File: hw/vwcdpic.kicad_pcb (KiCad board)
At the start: 2 copper layers, 14.6 x 13.1 mm, 12 parts, among them U1 PIC12F629, U2 LM78L05ACZ, U3 MC78L05ACH

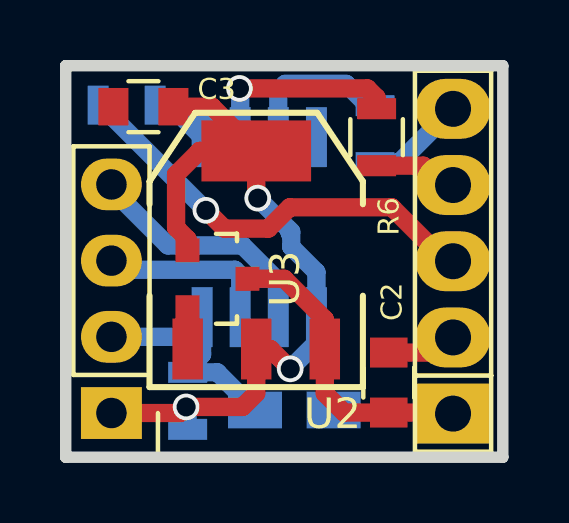
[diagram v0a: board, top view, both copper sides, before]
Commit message: update
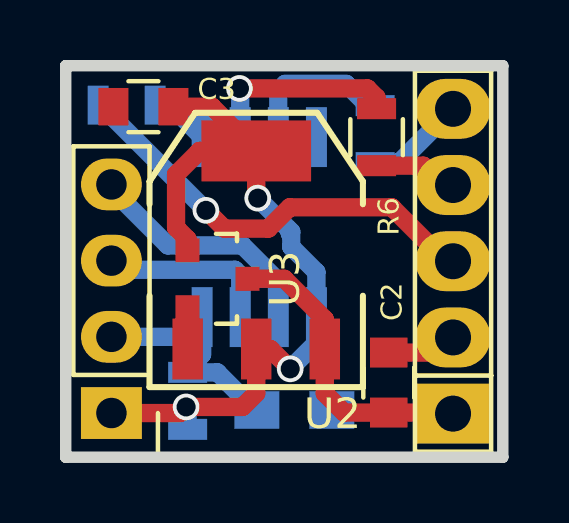
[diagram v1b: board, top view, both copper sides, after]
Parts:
- C1: value 1uF/6.3V -> 1uF/16V; footprint Capacitors_Tantalum_SMD:TantalC_SizeA_EIA-3216_Reflow -> Capacitors_SMD:C_0805_HandSoldering
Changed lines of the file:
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@@
-(kicad_pcb (version 4) (host pcbnew 0.201510080346+6253~30~ubuntu14.04.1-product)
+(kicad_pcb (version 4) (host pcbnew 0.201511080416+6302~30~ubuntu14.04.1-product)
   (general
     (links 26)
@@
       (net 10 ARCHOS))
   )
-  (module Capacitors_Tantalum_SMD:TantalC_SizeA_EIA-3216_Reflow (layer Back)
-    (at 145.3896 125.8824)
-    (descr "Tantal Cap. , Size A, EIA-3216, Reflow")
-    (tags "Tantal Capacitor Size-A EIA-3216 reflow")
-    (attr smd)
-    (fp_text reference C1 (at 2.2352 -1.6764 180) (layer B.SilkS)
-      (effects (font (size 0.7 0.7) (thickness 0.1)) (justify mirror))
-    )
-    (fp_text value 1uF/6.3V (at 0 -2.1) (layer B.Fab) hide
-      (effects (font (size 1 1) (thickness 0.15)) (justify mirror))
-    )
-    (fp_line (start 1.6 -0.9) (end -2.1 -0.9) (layer B.SilkS) (width 0.15))
-    (fp_line (start 1.6 0.9) (end -2.1 0.9) (layer B.SilkS) (width 0.15))
-    (fp_line (start -2.5 -1.2) (end 2.5 -1.2) (layer B.CrtYd) (width 0.05))
-    (fp_line (start 2.5 -1.2) (end 2.5 1.2) (layer B.CrtYd) (width 0.05))
-    (fp_line (start 2.5 1.2) (end -2.5 1.2) (layer B.CrtYd) (width 0.05))
-    (fp_line (start -2.5 1.2) (end -2.5 -1.2) (layer B.CrtYd) (width 0.05))
-    (pad 2 smd rect (at 1.31 0) (size 1.8 1.23) (layers Back B.Paste B.Mask)
-      (net 2 GND))
-    (pad 1 smd rect (at -1.31 0) (size 1.8 1.23) (layers Back B.Paste B.Mask)
-      (net 8 RESET))
-    (model Capacitors_Tantalum_SMD.3dshapes/TantalC_SizeA_EIA-3216_Reflow.wrl
-      (at (xyz 0 0 0))
-      (scale (xyz 1 1 1))
-      (rotate (xyz 0 0 180))
-    )
-  )
   (module Capacitors_SMD:C_0805 (layer Front)
     (at 148.5392 124.968 90)
@@
       (at (xyz 0 0 0))
       (scale (xyz 1 1 1))
+      (rotate (xyz 0 0 0))
+    )
+  )
+  (module Capacitors_SMD:C_0805_HandSoldering (layer Back)
+    (at 145.3896 125.8824)
+    (descr "Capacitor SMD 0805, hand soldering")
+    (tags "capacitor 0805")
+    (attr smd)
+    (fp_text reference C1 (at 0 2.1) (layer B.SilkS)
+      (effects (font (size 1 1) (thickness 0.15)) (justify mirror))
+    )
+    (fp_text value 1uF/16V (at 0 -2.1) (layer B.Fab)
+      (effects (font (size 1 1) (thickness 0.15)) (justify mirror))
+    )
+    (fp_line (start -2.3 1) (end 2.3 1) (layer B.CrtYd) (width 0.05))
+    (fp_line (start -2.3 -1) (end 2.3 -1) (layer B.CrtYd) (width 0.05))
+    (fp_line (start -2.3 1) (end -2.3 -1) (layer B.CrtYd) (width 0.05))
+    (fp_line (start 2.3 1) (end 2.3 -1) (layer B.CrtYd) (width 0.05))
+    (fp_line (start 0.5 0.85) (end -0.5 0.85) (layer B.SilkS) (width 0.15))
+    (fp_line (start -0.5 -0.85) (end 0.5 -0.85) (layer B.SilkS) (width 0.15))
+    (pad 1 smd rect (at -1.25 0) (size 1.5 1.25) (layers Back B.Paste B.Mask)
+      (net 8 RESET))
+    (pad 2 smd rect (at 1.25 0) (size 1.5 1.25) (layers Back B.Paste B.Mask)
+      (net 2 GND))
+    (model Capacitors_SMD.3dshapes/C_0805_HandSoldering.wrl
+      (at (xyz 0 0 0))
+      (scale (xyz 1 1 1))

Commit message: hw upgrade
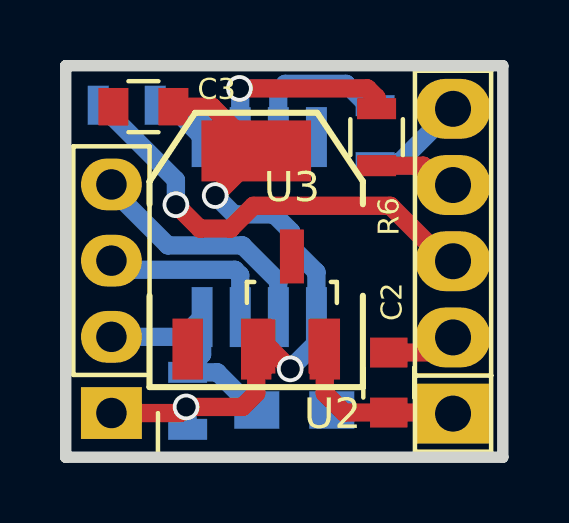
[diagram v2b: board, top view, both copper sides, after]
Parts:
- U3: footprint Housings_SOT-23_SOT-143_TSOT-6:SOT-23 -> TO_SOT_Packages_SMD:SOT-23_Handsoldering
- moved U3 2.59 mm to (145.3, 122.3), turned to 0 degrees
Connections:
- U3 pad 2: GND -> POWER_CTL
- U3 pad 3: POWER_CTL -> GND
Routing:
- net POWER_CTL: track 10.3 -> 6.18 mm
- net +5V: track 27.3 -> 23.5 mm
- net DataOut: track 15.4 -> 16.0 mm
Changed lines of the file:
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@@
-(kicad_pcb (version 4) (host pcbnew 0.201511080416+6302~30~ubuntu14.04.1-product)
+(kicad_pcb (version 4) (host pcbnew 0.201602161416+6560~42~ubuntu14.04.1-product)
   (general
     (links 26)
     (no_connects 0)
-    (area 137.579099 114.216179 152.529541 127.647701)
+    (area 134.285267 108.3056 162.509202 129.959)
     (thickness 1.6002)
     (drawings 6)
-    (tracks 94)
+    (tracks 89)
     (zones 0)
     (modules 12)
@@
       (hpglpenspeed 20)
       (hpglpendiameter 15)
-      (hpglpenoverlay 0)
       (psnegative false)
       (psa4output false)
@@
     )
   )
-  (module Housings_SOT-23_SOT-143_TSOT-6:SOT-23 (layer Front)
-    (at 142.82928 121.50852 270)
-    (descr "SOT-23, Standard")
-    (tags SOT-23)
-    (attr smd)
-    (fp_text reference U3 (at 0 -2.25 270) (layer F.SilkS)
-      (effects (font (size 1 1) (thickness 0.15)))
-    )
-    (fp_text value MC78L05ACH (at 0 2.3 270) (layer F.Fab)
-      (effects (font (size 1 1) (thickness 0.15)))
-    )
-    (fp_line (start -1.65 -1.6) (end 1.65 -1.6) (layer F.CrtYd) (width 0.05))
-    (fp_line (start 1.65 -1.6) (end 1.65 1.6) (layer F.CrtYd) (width 0.05))
-    (fp_line (start 1.65 1.6) (end -1.65 1.6) (layer F.CrtYd) (width 0.05))
-    (fp_line (start -1.65 1.6) (end -1.65 -1.6) (layer F.CrtYd) (width 0.05))
-    (fp_line (start 1.29916 -0.65024) (end 1.2509 -0.65024) (layer F.SilkS) (width 0.15))
-    (fp_line (start -1.49982 0.0508) (end -1.49982 -0.65024) (layer F.SilkS) (width 0.15))
-    (fp_line (start -1.49982 -0.65024) (end -1.2509 -0.65024) (layer F.SilkS) (width 0.15))
-    (fp_line (start 1.29916 -0.65024) (end 1.49982 -0.65024) (layer F.SilkS) (width 0.15))
-    (fp_line (start 1.49982 -0.65024) (end 1.49982 0.0508) (layer F.SilkS) (width 0.15))
-    (pad 1 smd rect (at -0.95 1.00076 270) (size 0.8001 0.8001) (layers Front F.Paste F.Mask)
-      (net 1 +5V))
-    (pad 2 smd rect (at 0.95 1.00076 270) (size 0.8001 0.8001) (layers Front F.Paste F.Mask)
-      (net 2 GND))
-    (pad 3 smd rect (at 0 -0.99822 270) (size 0.8001 0.8001) (layers Front F.Paste F.Mask)
-      (net 3 POWER_CTL))
-    (model TO_SOT_Packages_SMD.3dshapes/SOT-23.wrl
-      (at (xyz 0 0 0))
-      (scale (xyz 1 1 1))
-      (rotate (xyz 0 0 0))
-    )
-  )
   (module Capacitors_SMD:C_0805_HandSoldering (layer Back)
     (at 145.3896 125.8824)
@@
     )
   )
+  (module TO_SOT_Packages_SMD:SOT-23_Handsoldering (layer Front)
+    (at 145.30832 122.26544)
+    (descr "SOT-23, Handsoldering")
+    (tags SOT-23)
+    (attr smd)
+    (fp_text reference U3 (at 0 -3.81) (layer F.SilkS)
+      (effects (font (size 1 1) (thickness 0.15)))
+    )
+    (fp_text value MC78L05ACH (at 0 3.81) (layer F.Fab)
+      (effects (font (size 1 1) (thickness 0.15)))
+    )
+    (fp_line (start -1.49982 0.0508) (end -1.49982 -0.65024) (layer F.SilkS) (width 0.15))
+    (fp_line (start -1.49982 -0.65024) (end -1.2509 -0.65024) (layer F.SilkS) (width 0.15))
+    (fp_line (start 1.29916 -0.65024) (end 1.49982 -0.65024) (layer F.SilkS) (width 0.15))
+    (fp_line (start 1.49982 -0.65024) (end 1.49982 0.0508) (layer F.SilkS) (width 0.15))
+    (pad 1 smd rect (at -0.95 1.50114) (size 0.8001 1.80086) (layers Front F.Paste F.Mask)
+      (net 1 +5V))
+    (pad 2 smd rect (at 0.95 1.50114) (size 0.8001 1.80086) (layers Front F.Paste F.Mask)
+      (net 3 POWER_CTL))
+    (pad 3 smd rect (at 0 -1.50114) (size 0.8001 1.80086) (layers Front F.Paste F.Mask)
+      (net 2 GND))
+    (model TO_SOT_Packages_SMD.3dshapes/SOT-23_Handsoldering.wrl
+      (at (xyz 0 0 0))
+      (scale (xyz 1 1 1))
+      (rotate (xyz 0 0 0))
+    )
+  )
   (gr_line (start 152.33904 127.4572) (end 137.7696 127.4572) (angle 90) (layer Edge.Cuts) (width 0.381))
   (gr_line (start 152.33904 114.40668) (end 152.33904 127.4572) (angle 90) (layer Edge.Cuts) (width 0.381))
@@
     (arrow2b (pts (xy 137.7696 111.8108) (xy 138.896104 111.224379)))
   )
-  (segment (start 141.82852 120.55852) (end 141.82852 120.18772) (width 0.6096) (layer Front) (net 1))
-  (segment (start 141.82852 120.18772) (end 141.44752 119.80672) (width 0.6096) (layer Front) (net 1))
-  (segment (start 141.44752 119.80672) (end 141.44752 118.02872) (width 0.6096) (layer Front) (net 1))
-  (segment (start 141.44752 118.02872) (end 142.22984 117.2464) (width 0.6096) (layer Front) (net 1))
-  (segment (start 142.22984 117.2464) (end 144.1196 117.2464) (width 0.6096) (layer Front) (net 1))
+  (segment (start 144.1196 117.2464) (end 144.1196 117.36832) (width 0.6096) (layer Front) (net 1))
+  (segment (start 144.1196 117.36832) (end 142.75308 118.73484) (width 0.6096) (layer Front) (net 1))
+  (segment (start 143.383 119.36476) (end 144.71396 119.36476) (width 0.6096) (layer Back) (net 1))
+  (segment (start 142.75308 118.73484) (end 143.383 119.36476) (width 0.6096) (layer Back) (net 1))
+  (via (at 142.75308 118.73484) (size 0.889) (drill 0.635) (layers Front Back) (net 1))
   (segment (start 144.1196 123.8504) (end 144.59204 123.8504) (width 0.6096) (layer Front) (net 1))
   (segment (start 144.59204 123.8504) (end 145.25244 124.5108) (width 0.6096) (layer Front) (net 1))
@@
   (segment (start 145.288 120.4468) (end 145.288 119.9388) (width 0.6096) (layer Back) (net 1))
   (segment (start 146.1262 121.285) (end 145.288 120.4468) (width 0.6096) (layer Back) (net 1))
-  (segment (start 144.1196 118.7704) (end 144.1196 117.2464) (width 0.6096) (layer Front) (net 1))
-  (segment (start 144.1704 118.8212) (end 144.1196 118.7704) (width 0.6096) (layer Front) (net 1))
-  (via (at 144.1704 118.8212) (size 0.889) (drill 0.635) (layers Front Back) (net 1))
-  (segment (start 145.2372 119.888) (end 144.1704 118.8212) (width 0.6096) (layer Back) (net 1))
+  (segment (start 145.2372 119.888) (end 144.71396 119.36476) (width 0.6096) (layer Back) (net 1))
   (segment (start 144.1196 117.602) (end 144.1196 117.2464) (width 0.6096) (layer Front) (net 1))
   (segment (start 141.7828 125.7808) (end 143.6624 125.7808) (width 0.6096) (layer Front) (net 1))
@@
   (segment (start 150.17674 123.968) (end 150.68042 123.46432) (width 0.6096) (layer Front) (net 2))
   (segment (start 141.8336 123.7996) (end 141.8336 123.8504) (width 0.6096) (layer Front) (net 2))
-  (segment (start 146.4056 123.8504) (end 146.4056 122.8598) (width 0.6096) (layer Front) (net 3))
-  (segment (start 146.4056 122.8598) (end 145.05432 121.50852) (width 0.6096) (layer Front) (net 3))
-  (segment (start 145.05432 121.50852) (end 143.8275 121.50852) (width 0.6096) (layer Front) (net 3))
   (segment (start 148.5392 125.968) (end 150.6441 125.968) (width 0.6096) (layer Front) (net 3))
   (segment (start 150.6441 125.968) (end 150.68042 126.00432) (width 0.6096) (layer Front) (net 3))
@@
   (segment (start 141.2522 115.7224) (end 142.3162 116.7864) (width 0.6096) (layer Back) (net 4))
   (segment (start 140.7516 115.7224) (end 141.2522 115.7224) (width 0.6096) (layer Back) (net 4))
-  (segment (start 142.4432 119.2276) (end 142.44828 119.2276) (width 0.6096) (layer Front) (net 5))
-  (segment (start 143.05788 119.8372) (end 144.526 119.8372) (width 0.6096) (layer Front) (net 5))
-  (segment (start 142.44828 119.2276) (end 143.05788 119.8372) (width 0.6096) (layer Front) (net 5))
-  (segment (start 138.938 115.7224) (end 142.4432 119.2276) (width 0.6096) (layer Back) (net 5))
-  (via (at 142.4432 119.2276) (size 0.889) (drill 0.635) (layers Front Back) (net 5))
-  (segment (start 150.43912 120.92432) (end 148.6408 119.126) (width 0.6096) (layer Front) (net 5))
-  (segment (start 145.2372 119.126) (end 144.526 119.8372) (width 0.6096) (layer Front) (net 5))
-  (segment (start 148.6408 119.126) (end 145.2372 119.126) (width 0.6096) (layer Front) (net 5))
+  (segment (start 150.68042 120.92432) (end 150.43912 120.92432) (width 0.6096) (layer Front) (net 5))
+  (segment (start 150.43912 120.92432) (end 148.59 119.0752) (width 0.6096) (layer Front) (net 5))
+  (segment (start 144.02816 119.0752) (end 143.26616 119.8372) (width 0.6096) (layer Front) (net 5))
+  (segment (start 148.59 119.0752) (end 144.02816 119.0752) (width 0.6096) (layer Front) (net 5))
+  (segment (start 138.8516 115.7224) (end 138.94816 115.7224) (width 0.6096) (layer Back) (net 5))
+  (segment (start 138.94816 115.7224) (end 141.44244 118.21668) (width 0.6096) (layer Back) (net 5))
+  (segment (start 142.24 119.8372) (end 143.26616 119.8372) (width 0.6096) (layer Front) (net 5))
+  (segment (start 141.44244 119.03964) (end 142.24 119.8372) (width 0.6096) (layer Front) (net 5))
+  (via (at 141.44244 119.03964) (size 0.889) (drill 0.635) (layers Front Back) (net 5))
+  (segment (start 141.44244 118.21668) (end 141.44244 119.03964) (width 0.6096) (layer Back) (net 5))
   (segment (start 138.8516 115.7224) (end 138.938 115.7224) (width 0.6096) (layer Back) (net 5))
-  (segment (start 150.68042 120.92432) (end 150.43912 120.92432) (width 0.6096) (layer Front) (net 5))
   (segment (start 150.68042 120.92432) (end 150.54072 120.92432) (width 0.6096) (layer Front) (net 5))
   (segment (start 150.68042 120.92432) (end 150.48992 120.92432) (width 0.6096) (layer Front) (net 5))
